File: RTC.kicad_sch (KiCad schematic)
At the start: 2 parts, among them U2 DS1307ZN+, Y2 32.768 kHz

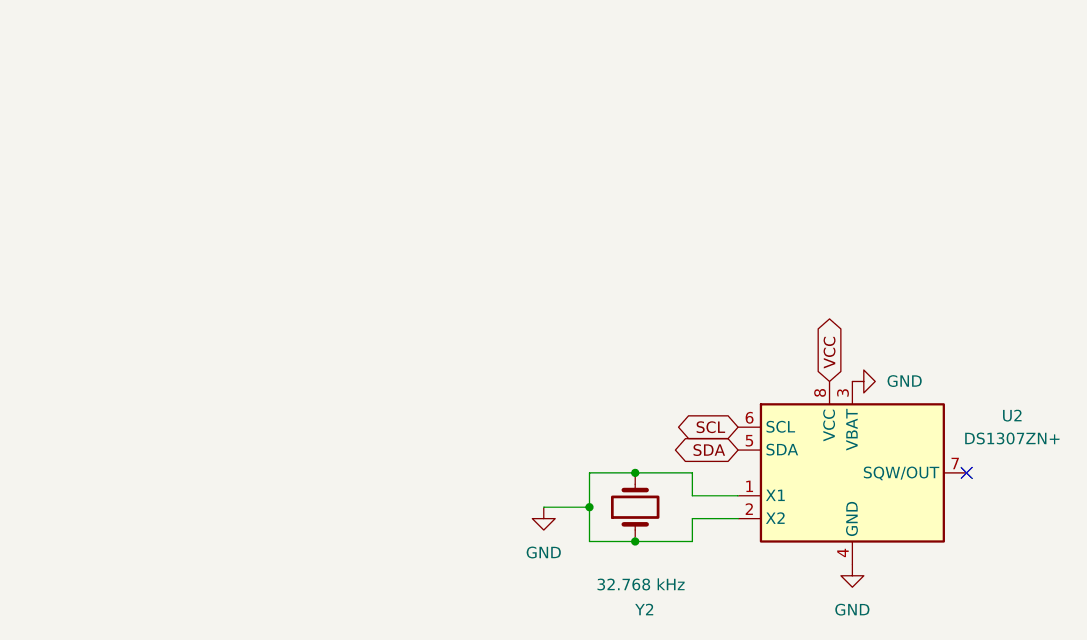
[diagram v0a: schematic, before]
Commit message: Draw basic inital schematic
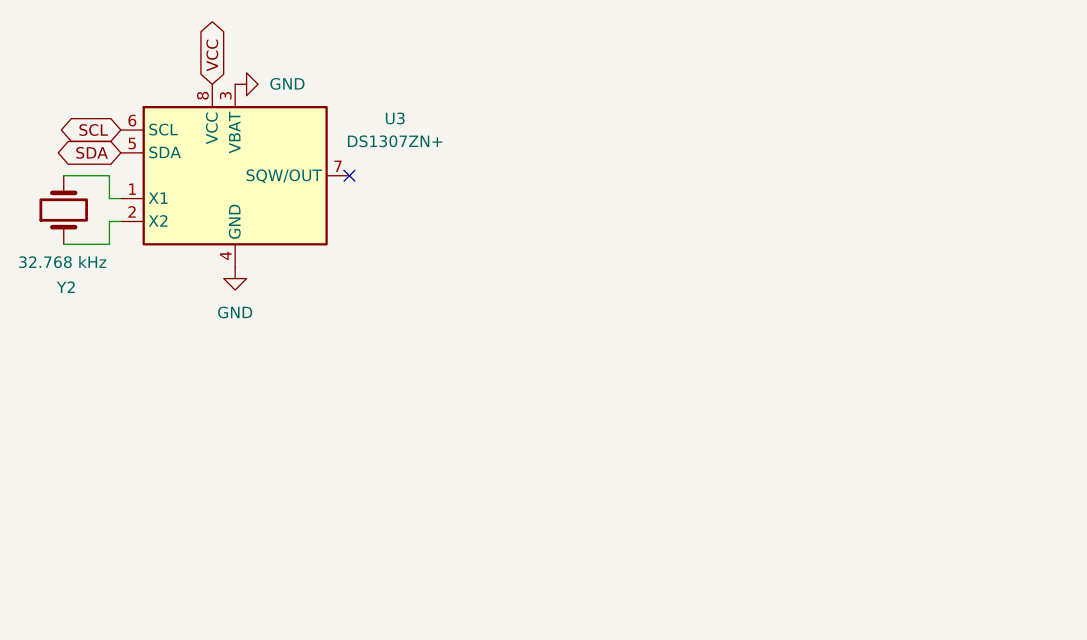
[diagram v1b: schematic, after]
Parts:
- renumbered U2 to U3
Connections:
- net GND: no longer U3.1 (X1), U3.2 (X2), Y2.1, Y2.2
- new net: U3.2 (X2), Y2.1
- new net: U3.1 (X1), Y2.2
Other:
- moved on the sheet: U3, Y2
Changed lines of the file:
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@@
 	(generator_version "8.0")
 	(paper "A4")
-	(junction
-		(at 80.01 69.85)
-		(diameter 0)
-		(color 0 0 0 0)
-	)
-	(junction
-		(at 85.09 73.66)
-		(diameter 0)
-		(color 0 0 0 0)
-	)
-	(junction
-		(at 85.09 66.04)
-		(diameter 0)
-		(color 0 0 0 0)
-	)
 	(no_connect
-		(at 121.92 66.04)
-	)
-	(wire
-		(pts
-			(xy 74.93 69.85) (xy 80.01 69.85)
-		)
-		(stroke
-			(width 0)
-			(type default)
-		)
-	)
-	(wire
-		(pts
-			(xy 85.09 66.04) (xy 91.44 66.04)
-		)
-		(stroke
-			(width 0)
-			(type default)
-		)
-	)
-	(wire
-		(pts
-			(xy 91.44 68.58) (xy 91.44 66.04)
-		)
-		(stroke
-			(width 0)
-			(type default)
-		)
-	)
-	(wire
-		(pts
-			(xy 96.52 71.12) (xy 91.44 71.12)
-		)
-		(stroke
-			(width 0)
-			(type default)
-		)
-	)
-	(wire
-		(pts
-			(xy 80.01 66.04) (xy 85.09 66.04)
-		)
-		(stroke
-			(width 0)
-			(type default)
-		)
-	)
-	(wire
-		(pts
-			(xy 96.52 68.58) (xy 91.44 68.58)
-		)
-		(stroke
-			(width 0)
-			(type default)
-		)
-	)
-	(wire
-		(pts
-			(xy 91.44 71.12) (xy 91.44 73.66)
-		)
-		(stroke
-			(width 0)
-			(type default)
-		)
-	)
-	(wire
-		(pts
-			(xy 85.09 73.66) (xy 91.44 73.66)
-		)
-		(stroke
-			(width 0)
-			(type default)
-		)
-	)
-	(wire
-		(pts
-			(xy 80.01 66.04) (xy 80.01 69.85)
-		)
-		(stroke
-			(width 0)
-			(type default)
-		)
-	)
-	(wire
-		(pts
-			(xy 85.09 73.66) (xy 80.01 73.66)
-		)
-		(stroke
-			(width 0)
-			(type default)
-		)
-	)
-	(wire
-		(pts
-			(xy 80.01 69.85) (xy 80.01 73.66)
+		(at 53.34 33.02)
+	)
+	(wire
+		(pts
+			(xy 26.67 35.56) (xy 26.67 33.02)
+		)
+		(stroke
+			(width 0)
+			(type default)
+		)
+	)
+	(wire
+		(pts
+			(xy 27.94 38.1) (xy 26.67 38.1)
+		)
+		(stroke
+			(width 0)
+			(type default)
+		)
+	)
+	(wire
+		(pts
+			(xy 21.59 40.64) (xy 26.67 40.64)
+		)
+		(stroke
+			(width 0)
+			(type default)
+		)
+	)
+	(wire
+		(pts
+			(xy 21.59 33.02) (xy 26.67 33.02)
+		)
+		(stroke
+			(width 0)
+			(type default)
+		)
+	)
+	(wire
+		(pts
+			(xy 27.94 35.56) (xy 26.67 35.56)
+		)
+		(stroke
+			(width 0)
+			(type default)
+		)
+	)
+	(wire
+		(pts
+			(xy 26.67 38.1) (xy 26.67 40.64)
 		)
 		(stroke
@@
 	(global_label "SCL"
 		(shape bidirectional)
-		(at 96.52 60.96 180)
+		(at 27.94 27.94 180)
 		(fields_autoplaced yes)
 		(effects
@@
 		)
 		(property "Intersheetrefs" "${INTERSHEET_REFS}"
-			(at 88.9159 60.96 0)
+			(at 20.3359 27.94 0)
 			(effects
 				(font
@@
 	(global_label "VCC"
 		(shape bidirectional)
-		(at 106.68 55.88 90)
+		(at 38.1 22.86 90)
 		(fields_autoplaced yes)
 		(effects
@@
 		)
 		(property "Intersheetrefs" "${INTERSHEET_REFS}"
-			(at 106.68 48.1549 90)
+			(at 38.1 15.1349 90)
 			(effects
 				(font
@@
 	(global_label "SDA"
 		(shape bidirectional)
-		(at 96.52 63.5 180)
+		(at 27.94 30.48 180)
 		(fields_autoplaced yes)
 		(effects
@@
 		)
 		(property "Intersheetrefs" "${INTERSHEET_REFS}"
-			(at 88.8554 63.5 0)
+			(at 20.2754 30.48 0)
 			(effects
 				(font
@@
 	(symbol
 		(lib_id "power:GND")
-		(at 109.22 55.88 90)
+		(at 40.64 22.86 90)
 		(unit 1)
 		(exclude_from_sim no)
@@
 		(dnp no)
 		(fields_autoplaced yes)
-		(property "Reference" "#PWR04"
-			(at 115.57 55.88 0)
+		(property "Reference" "#PWR015"
+			(at 46.99 22.86 0)
 			(effects
 				(font
@@
 		)
 		(property "Value" "GND"
-			(at 113.03 55.8799 90)
+			(at 44.45 22.8599 90)
 			(effects
 				(font
@@
 		)
 		(property "Footprint" ""
-			(at 109.22 55.88 0)
+			(at 40.64 22.86 0)
 			(effects
 				(font
@@
 		)
 		(property "Datasheet" ""
-			(at 109.22 55.88 0)
+			(at 40.64 22.86 0)
 			(effects
 				(font
@@
 		)
 		(property "Description" "Power symbol creates a global label with name \"GND\" , ground"
-			(at 109.22 55.88 0)
+			(at 40.64 22.86 0)
 			(effects
 				(font
@@
 			(project "plokkskeem"
 				(path "/a526e2f2-17cc-4dbb-8268-7175c0e116d3/320a11b5-8e7b-40af-9ca3-15dbc2f11b10"
-					(reference "#PWR04")
-					(unit 1)
-				)
-			)
-		)
-	)
-	(symbol
-		(lib_id "power:GND")
-		(at 74.93 69.85 0)
-		(unit 1)
-		(exclude_from_sim no)
-		(in_bom yes)
-		(on_board yes)
-		(dnp no)
-		(fields_autoplaced yes)
-		(property "Reference" "#PWR03"
-			(at 74.93 76.2 0)
-			(effects
-				(font
-					(size 1.27 1.27)
-				)
-				(hide yes)
-			)
-		)
-		(property "Value" "GND"
-			(at 74.93 74.93 0)
-			(effects
-				(font
-					(size 1.27 1.27)
-				)
-			)
-		)
-		(property "Footprint" ""
-			(at 74.93 69.85 0)
-			(effects
-				(font
-					(size 1.27 1.27)
-				)
-				(hide yes)
-			)
-		)
-		(property "Datasheet" ""
-			(at 74.93 69.85 0)
-			(effects
-				(font
-					(size 1.27 1.27)
-				)
-				(hide yes)
-			)
-		)
-		(property "Description" "Power symbol creates a global label with name \"GND\" , ground"
-			(at 74.93 69.85 0)
-			(effects
-				(font
-					(size 1.27 1.27)
-				)
-				(hide yes)
-			)
-		)
-		(pin "1"
-		)
-		(instances
-			(project "plokkskeem"
-				(path "/a526e2f2-17cc-4dbb-8268-7175c0e116d3/320a11b5-8e7b-40af-9ca3-15dbc2f11b10"
-					(reference "#PWR03")
+					(reference "#PWR015")
 					(unit 1)
 				)
@@
 	(symbol
 		(lib_id "Device:Crystal")
-		(at 85.09 69.85 90)
+		(at 21.59 36.83 90)
 		(unit 1)
 		(exclude_from_sim no)
@@
 		(dnp no)
 		(property "Reference" "Y2"
-			(at 85.09 81.28 90)
+			(at 20.828 45.466 90)
 			(effects
 				(font
@@
 		)
 		(property "Value" "32.768 kHz"
-			(at 80.772 78.486 90)
+			(at 16.51 42.672 90)
 			(effects
 				(font
@@
 		)
 		(property "Footprint" ""
-			(at 85.09 69.85 0)
+			(at 21.59 36.83 0)
 			(effects
 				(font
@@
 		)
 		(property "Datasheet" "~"
-			(at 85.09 69.85 0)
+			(at 21.59 36.83 0)
 			(effects
 				(font
@@
 		)
 		(property "Description" "Two pin crystal"
-			(at 85.09 69.85 0)
+			(at 21.59 36.83 0)
 			(effects
 				(font
@@
 	(symbol
 		(lib_id "Timer_RTC:DS1307ZN+")
-		(at 109.22 66.04 0)
+		(at 40.64 33.02 0)
 		(unit 1)
 		(exclude_from_sim no)
@@
 		(on_board yes)
 		(dnp no)
-		(property "Reference" "U2"
-			(at 127 59.7214 0)
+		(property "Reference" "U3"
+			(at 58.42 26.7014 0)
 			(effects
 				(font
@@
 		)
 		(property "Value" "DS1307ZN+"
-			(at 127 62.2614 0)
+			(at 58.42 29.2414 0)
 			(effects
 				(font
@@
 		)
 		(property "Footprint" "Package_SO:SOIC-8_3.9x4.9mm_P1.27mm"
-			(at 109.22 78.74 0)
+			(at 40.64 45.72 0)
 			(effects
 				(font
@@
 		)
 		(property "Datasheet" "https://datasheets.maximintegrated.com/en/ds/DS1307.pdf"
-			(at 109.22 66.04 0)
+			(at 40.64 33.02 0)
 			(effects
 				(font
@@
 		)
 		(property "Description" "64 x 8, Serial, I2C Real-time clock, 4.5V to 5.5V VCC, -40°C to +85°C, SOIC-8"
-			(at 109.22 66.04 0)
+			(at 40.64 33.02 0)
 			(effects
 				(font
@@
 			(project "plokkskeem"
 				(path "/a526e2f2-17cc-4dbb-8268-7175c0e116d3/320a11b5-8e7b-40af-9ca3-15dbc2f11b10"
-					(reference "U2")
+					(reference "U3")
 					(unit 1)
 				)
@@
 	(symbol
 		(lib_id "power:GND")
-		(at 109.22 76.2 0)
+		(at 40.64 43.18 0)
 		(unit 1)
 		(exclude_from_sim no)
@@
 		(fields_autoplaced yes)
 		(property "Reference" "#PWR016"
-			(at 109.22 82.55 0)
+			(at 40.64 49.53 0)
 			(effects
 				(font
@@
 		)
 		(property "Value" "GND"
-			(at 109.22 81.28 0)
+			(at 40.64 48.26 0)
 			(effects
 				(font
@@
 		)
 		(property "Footprint" ""
-			(at 109.22 76.2 0)
+			(at 40.64 43.18 0)
 			(effects
 				(font
@@
 		)
 		(property "Datasheet" ""
-			(at 109.22 76.2 0)
+			(at 40.64 43.18 0)
 			(effects
 				(font
@@
 		)
 		(property "Description" "Power symbol creates a global label with name \"GND\" , ground"
-			(at 109.22 76.2 0)
-			(effects
-				(font
+			(at 40.64 43.18 0)
+			(effects
+				(font
